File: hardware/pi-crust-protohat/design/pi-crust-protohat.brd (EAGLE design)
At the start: 65 x 56.5 mm, 13 parts, among them U1 EEPROM24

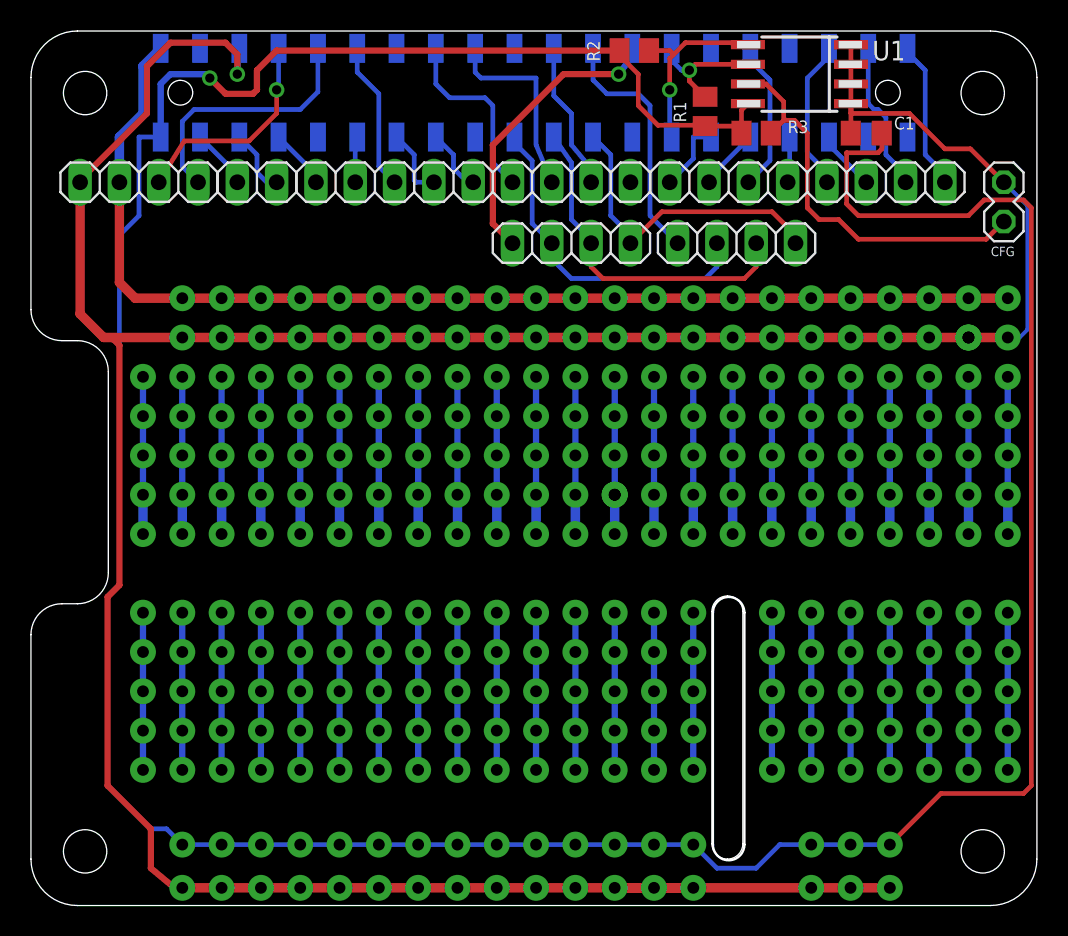
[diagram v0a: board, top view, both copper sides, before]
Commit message: update hardware designs for plus and protohat
update hardware designs for plus and protohat
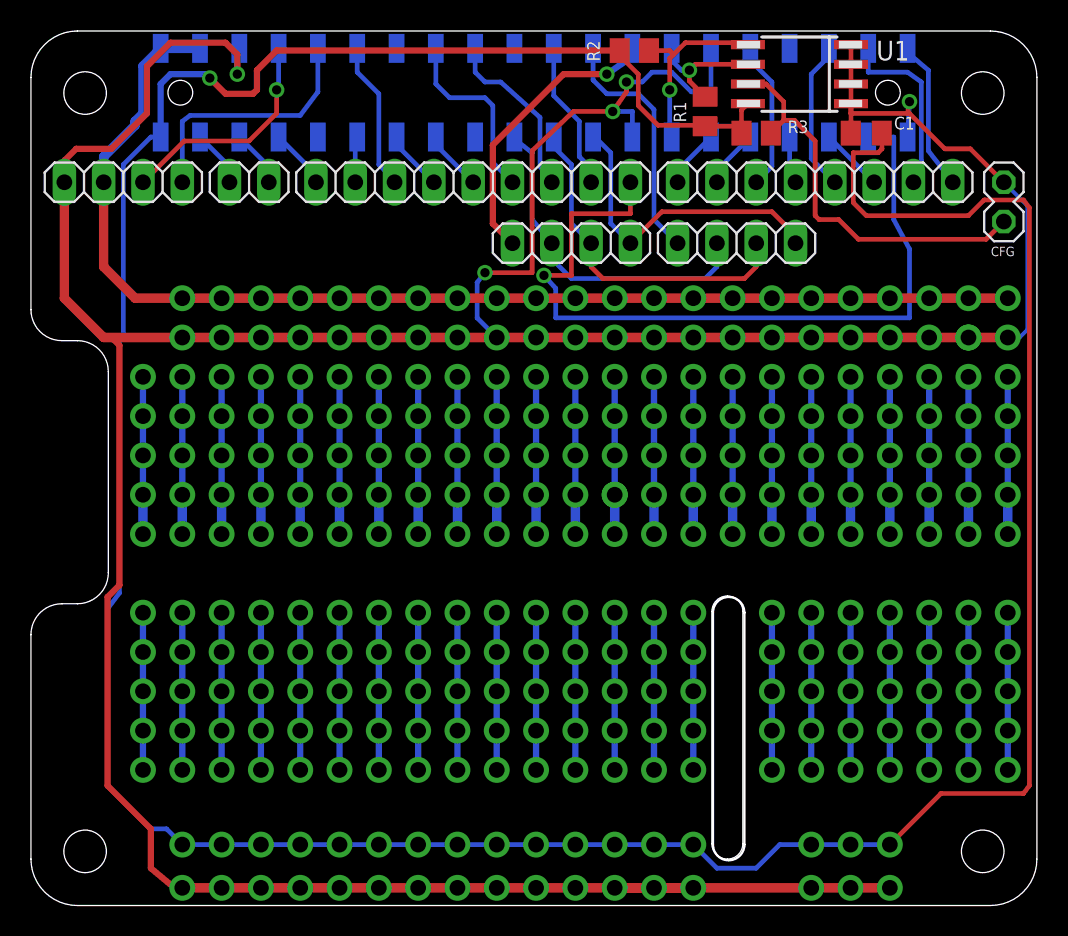
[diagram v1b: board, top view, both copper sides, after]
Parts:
- moved JP6 1.02 mm to (5.84, -10.3)
- moved JP11 0.51 mm to (50.5, -10.3)
- moved JP1 0.51 mm to (14.0, -10.3)
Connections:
- removed net N$14: JP5.9
- net +5V: now also U$1.P4
- net GND: now also U$1.P25, U$1.P30, U$1.P39
- net GPIO_26: now also JP5.9
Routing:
- net GPIO_26: track 0.00 -> 51.1 mm, vias 0 -> 1
- net GND: track 207.1 -> 248.6 mm, vias 41 -> 45
- net +5V: track 74.1 -> 77.4 mm
- net GPIO_20: track 9.80 -> 11.7 mm
- net +3V3: track 214.6 -> 213.1 mm
- net GPIO_24: track 12.6 -> 11.3 mm
- net GPIO_27: track 5.10 -> 3.92 mm
- net GPIO_05: track 4.70 -> 3.82 mm
- net UART_TX: track 14.1 -> 14.7 mm
- net I2C_SCL: track 4.29 -> 3.71 mm
- net SPI_MISO: track 22.7 -> 22.2 mm
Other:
- board text added: "26"
